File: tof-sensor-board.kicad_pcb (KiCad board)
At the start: 2 copper layers, 20.8 x 16.8 mm, 30 parts, among them U1 STM32F302K8U6, U2 LTC2875, U3 MCP1703, U4 VL53L0X, X1 16MHz

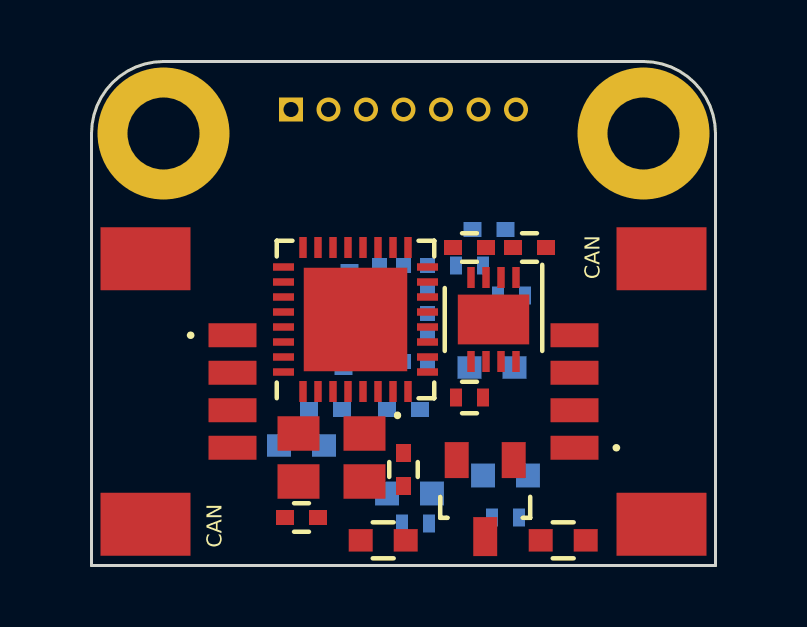
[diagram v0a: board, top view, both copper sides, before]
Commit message: routing
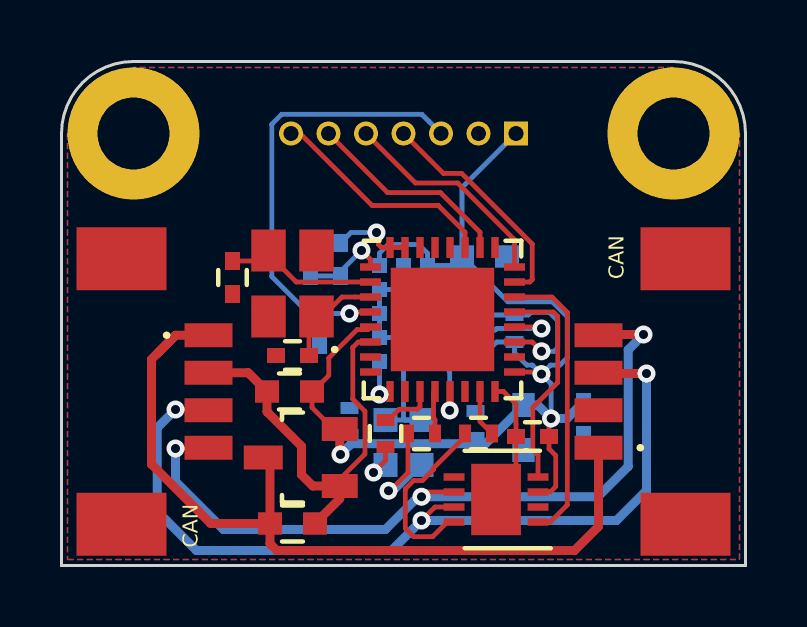
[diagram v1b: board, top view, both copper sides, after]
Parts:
- removed _M2: VAL**, _mech:_M2
- added MEC2: MEC, _mech:_M2, F.Cu at (59.3, 45.0)
- C2: moved to B.Cu
- MEC1: renamed from _M2; value VAL** -> MEC
- R6, R7: moved to F.Cu
- R8: value 0 -> 1k
- moved C4 9.04 mm to (46.3, 57.0)
- moved C9 8.32 mm to (44.3, 48.8), turned to 270 degrees
- moved CONN1 7.54 mm to (53.8, 44.0), turned to 180 degrees
- moved C1 7.42 mm to (54.0, 53.8), turned to 270 degrees
- moved C7 7.04 mm to (56.0, 53.5), turned to 270 degrees
- moved R9 6.56 mm to (48.2, 53.6), turned to 90 degrees
- moved C11 6.30 mm to (54.3, 54.1), turned to 180 degrees
- moved U3 6.27 mm to (46.6, 54.8), turned to 90 degrees
- moved U2 6.00 mm to (53.1, 56.2), turned to 180 degrees
- moved X1 5.94 mm to (46.3, 49.0), turned to 90 degrees
- moved C13 5.88 mm to (46.9, 48.2), turned to 90 degrees
- moved C5 5.86 mm to (46.2, 52.6)
- moved R3 5.77 mm to (53.7, 50.5)
- moved C8 5.30 mm to (46.3, 51.4), turned to 180 degrees
- moved R4 4.83 mm to (52.6, 51.0), turned to 90 degrees
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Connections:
- U1 pad 10: /XSHUT -> (no net)
- U1 pad 11: /GPIO1 -> /Proximity
- U1 pad 12: (no net) -> /Error
- U1 pad 13: (no net) -> /GPIO1
- U1 pad 15: (no net) -> /CAN_SPEED
- U1 pad 7: /Proximity -> (no net)
- U1 pad 8: /Error -> (no net)
- U1 pad 9: /CAN_SPEED -> /XSHUT
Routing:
- net VCC: track 0.00 -> 42.7 mm, vias 0 -> 4
- net Net-(CONN2-Pad3): track 0.00 -> 29.2 mm, vias 0 -> 3
- net +5V: track 0.00 -> 28.3 mm
- net GND: track 0.00 -> 28.1 mm, vias 0 -> 1
- net Net-(CONN2-Pad4): track 0.00 -> 26.1 mm, vias 0 -> 3
- net /STM32_NRST: track 0.00 -> 14.9 mm, vias 0 -> 1
- net /CAN_TX: track 0.00 -> 9.60 mm
- net /UART2_RX: track 0.00 -> 7.67 mm
- net /STM32_SWDIO: track 0.00 -> 7.63 mm
- net /I2C_SCL: track 0.00 -> 7.37 mm, vias 0 -> 1
- net /STM32_SWCLK: track 0.00 -> 7.32 mm
- net /CAN_RX: track 0.00 -> 7.27 mm
- net /UART2_TX: track 0.00 -> 6.92 mm
- net Net-(R8-Pad1): track 0.00 -> 6.10 mm
- net Net-(C9-Pad1): track 0.00 -> 5.25 mm
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- added copper zone on B.Cu, net GND
- added copper zone on F.Cu, net GND
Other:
- board size 20.8 x 16.8 mm -> 22.8 x 16.8 mm
